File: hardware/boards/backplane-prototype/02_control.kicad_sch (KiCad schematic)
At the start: 14 parts, among them J10 TC2030-IDC-NL SWD, U1 STM32C092GCU6

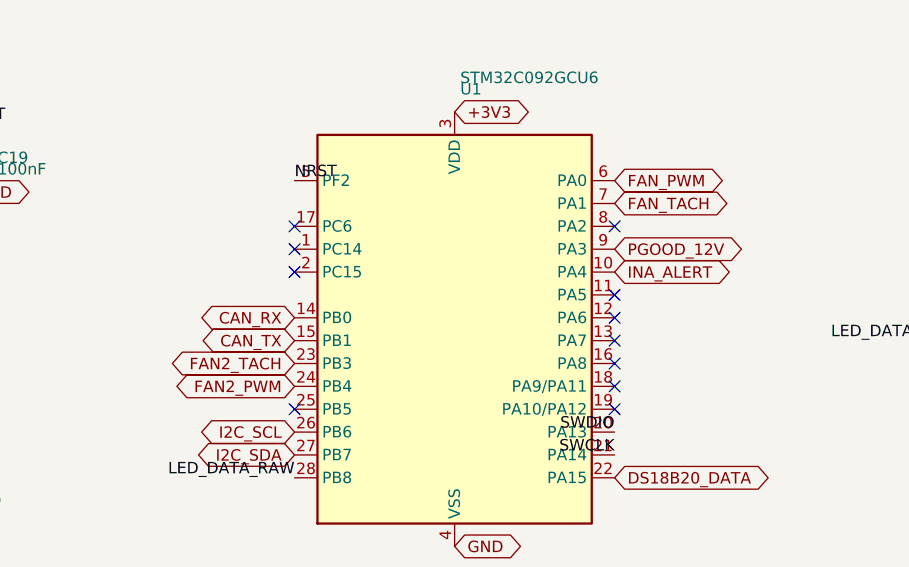
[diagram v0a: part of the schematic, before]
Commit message: checkpoint before fan pin swap review
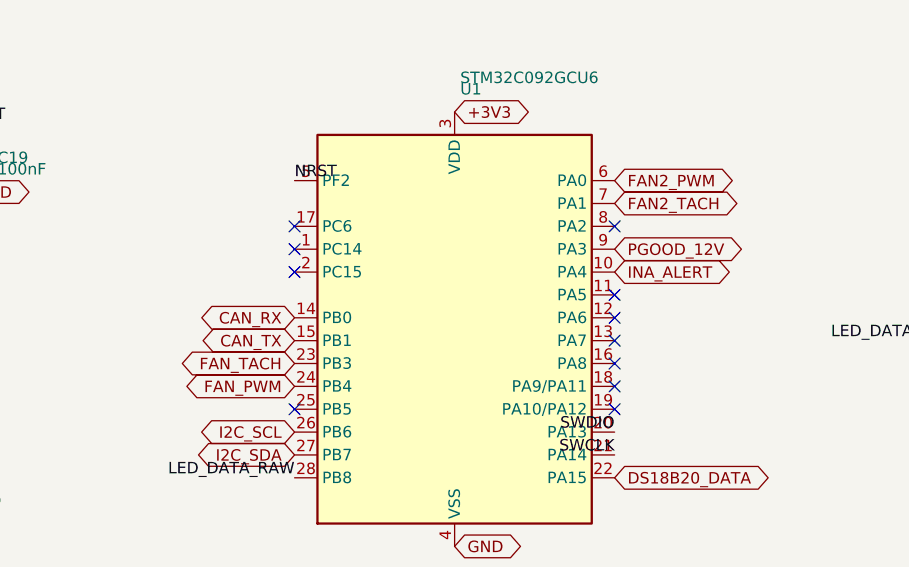
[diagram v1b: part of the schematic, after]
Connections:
- net FAN2_PWM: now also U1.6 (PA0); no longer U1.24 (PB4)
- net FAN2_TACH: now also U1.7 (PA1); no longer U1.23 (PB3)
- net FAN_PWM: now also U1.24 (PB4); no longer U1.6 (PA0)
- net FAN_TACH: now also U1.23 (PB3); no longer U1.7 (PA1)
